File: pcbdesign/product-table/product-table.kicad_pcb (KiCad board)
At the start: 2 copper layers, 60 x 57 mm, 26 parts, among them U1 LM1117-3.3

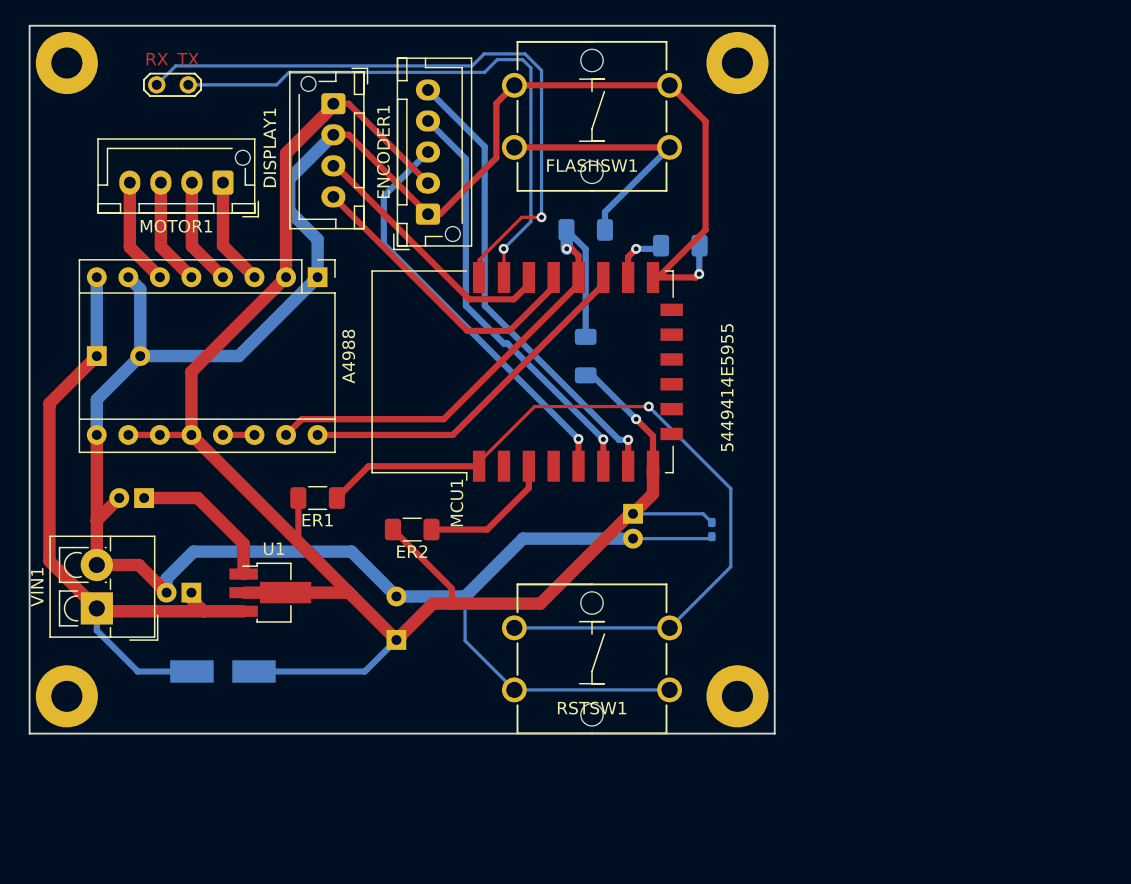
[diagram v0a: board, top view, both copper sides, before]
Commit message: Update all
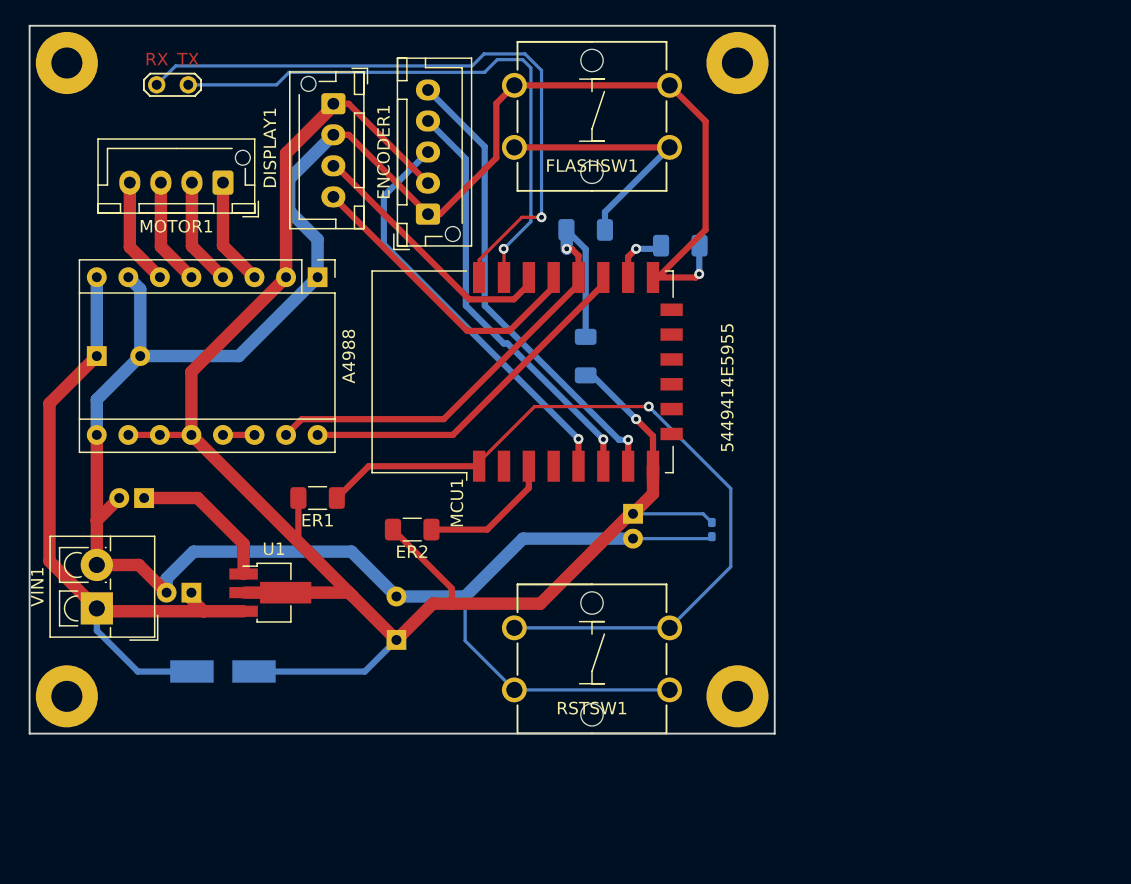
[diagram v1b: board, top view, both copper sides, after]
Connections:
- RSTSW1 pad 2: /esp8266/RST -> GND
- RSTSW1 pad 3: GND -> /esp8266/RST
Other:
- net class JLCPCB added: clearance 0.2, trace_width 0.25, via_dia 0.8, via_drill 0.4
- rule trace_min: 0.2 -> 0.127
- rule via_min_drill: 0.3 -> 0.2
- rule via_min_size: 0.4 -> 0.45

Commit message: Updated pcb design
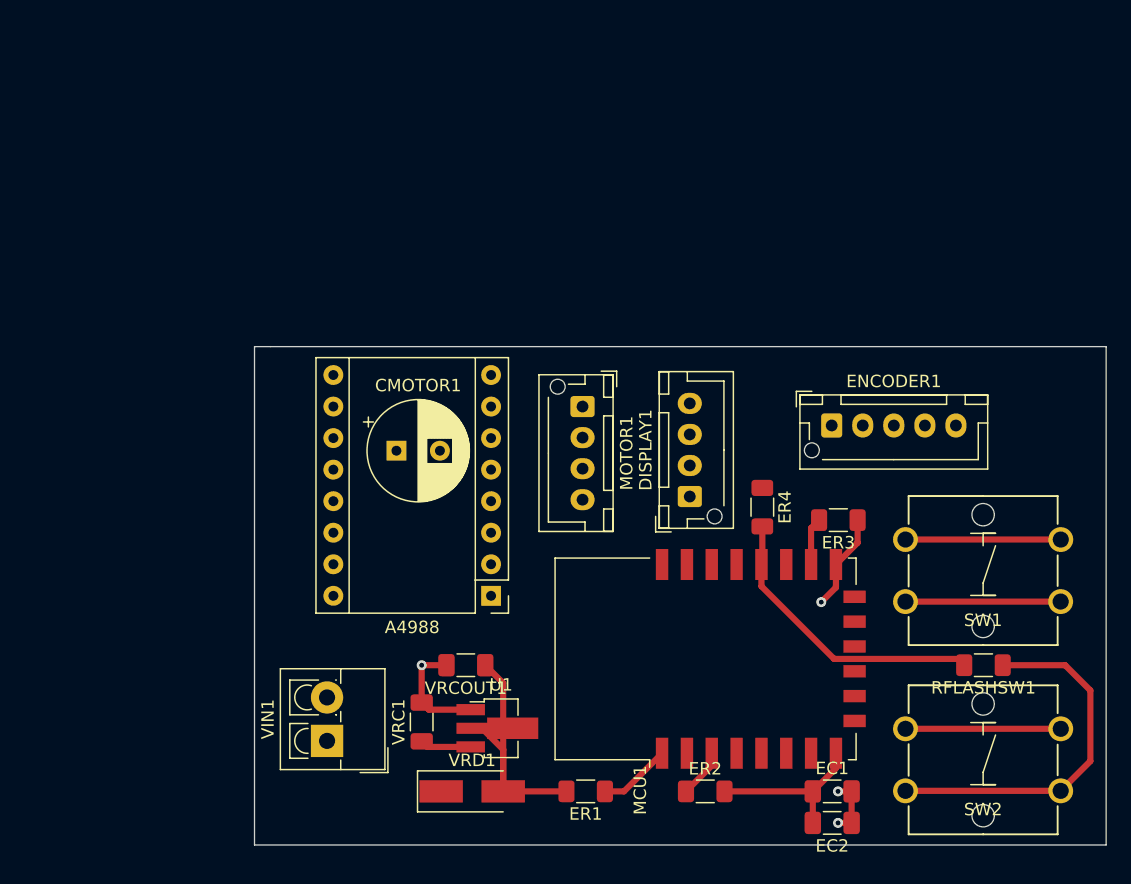
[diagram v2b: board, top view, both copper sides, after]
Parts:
- removed FLASHSW1, RSTSW1: SW_Push_Dual, custom-footprints:SW_PUSH_Omron_B3F-4055
- removed REF**: TestPoint_2Pads_Pitch2.54mm_Drill0.8mm, TestPoint:TestPoint_2Pads_Pitch2.54mm_Drill0.8mm
- removed REF** (x4): MountingHole_2.5mm_Pad, MountingHole:MountingHole_2.5mm_Pad
- removed VRCADJ1: 10uF, Capacitor_THT:CP_Radial_D5.0mm_P2.00mm
- added SW1: Omron-B3F-4055, custom-footprints:SW_PUSH_Omron_B3F-4055, F.Cu at (176.8, 118.9)
- added SW2: Omron-B3F-4055, custom-footprints:SW_PUSH_Omron_B3F-4055, F.Cu at (176.8, 134.1)
- CMOTOR1, ER3, ER4, VRD1: moved to F.Cu
- EC1, VRC1: footprint Capacitor_THT:CP_Radial_D5.0mm_P2.00mm -> Capacitor_SMD:C_1206_3216Metric_Pad1.33x1.80mm_HandSolder; moved to F.Cu
- EC2: footprint Capacitor_SMD:C_0402_1005Metric_Pad0.74x0.62mm_HandSolder -> Capacitor_SMD:C_1206_3216Metric_Pad1.33x1.80mm_HandSolder; moved to F.Cu
- RFLASHSW1: value 10K -> 100; moved to F.Cu
- VRCOUT1: value 100uF -> 10uF; footprint Capacitor_THT:CP_Radial_D8.0mm_P3.50mm -> Capacitor_SMD:C_1206_3216Metric_Pad1.33x1.80mm_HandSolder; moved to F.Cu
- moved RFLASHSW1 47.5 mm to (176.8, 126.5)
- moved DISPLAY1 42.7 mm to (153.2, 112.9), turned to 90 degrees
- moved ENCODER1 36.7 mm to (164.6, 107.2), turned to 0 degrees
- moved MOTOR1 34.1 mm to (144.5, 105.7), turned to 270 degrees
- moved ER1 32.0 mm to (144.8, 136.7)
- moved ER2 31.6 mm to (154.4, 136.7), turned to 0 degrees
- moved A4988 29.2 mm to (137.2, 120.9), turned to 180 degrees
- moved EC1 27.5 mm to (164.6, 136.7), turned to 0 degrees
- moved MCU1 27.4 mm to (154.4, 126.0)
- moved EC2 25.5 mm to (164.6, 139.2), turned to 180 degrees
- moved ER3 25.5 mm to (165.1, 114.8)
- moved CMOTOR1 25.3 mm to (129.5, 109.2)
- moved VRD1 22.3 mm to (135.6, 136.7)
- moved VIN1 21.4 mm to (124.0, 132.6)
- moved U1 21.3 mm to (137.7, 131.6)
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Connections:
- U1 pad 1: Net-(U1-Pad1) -> GND
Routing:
- net GND: track 197.4 -> 46.7 mm, vias 1 -> 4
- net +3V3: track 159.0 -> 36.0 mm, vias 1 -> 0
- net /esp8266/ESPTX: track 52.3 -> 0.00 mm, vias 1 -> 0
- net +12V: track 54.5 -> 4.13 mm
- net /esp8266/ESPRX: track 46.5 -> 0.00 mm, vias 1 -> 0
- net /esp8266/RST: track 63.5 -> 18.4 mm, vias 1 -> 0
- net /GPIO13: track 37.4 -> 0.00 mm, vias 1 -> 0
- net /GPIO12: track 33.8 -> 0.00 mm, vias 1 -> 0
- net /GPIO14: track 33.3 -> 0.00 mm, vias 1 -> 0
- net /GPIO2: track 28.6 -> 0.00 mm
- net /GPIO4: track 24.4 -> 0.00 mm
- net /GPIO5: track 21.2 -> 0.00 mm
- net /GPIO0: track 42.8 -> 23.8 mm, vias 1 -> 0
- net Net-(U1-Pad1): track 12.0 -> 0.00 mm
- net Net-(A4988-Pad3): track 8.67 -> 0.00 mm
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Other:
- board size 60 x 57 mm -> 68.6 x 40.1 mm
- board text removed: "5449414E5955"
- board text removed: "RX"
- board text removed: "TX"
